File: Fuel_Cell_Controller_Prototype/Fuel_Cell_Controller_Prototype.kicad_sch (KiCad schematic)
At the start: 43 parts, among them J3 6POS MOLEX, Q1 NMOS, Q2 NMOS, U3 MAX14572, U4 MAX14572, U6 SHT31-DIS, U7 BUF602xD, U8 BUF602xD

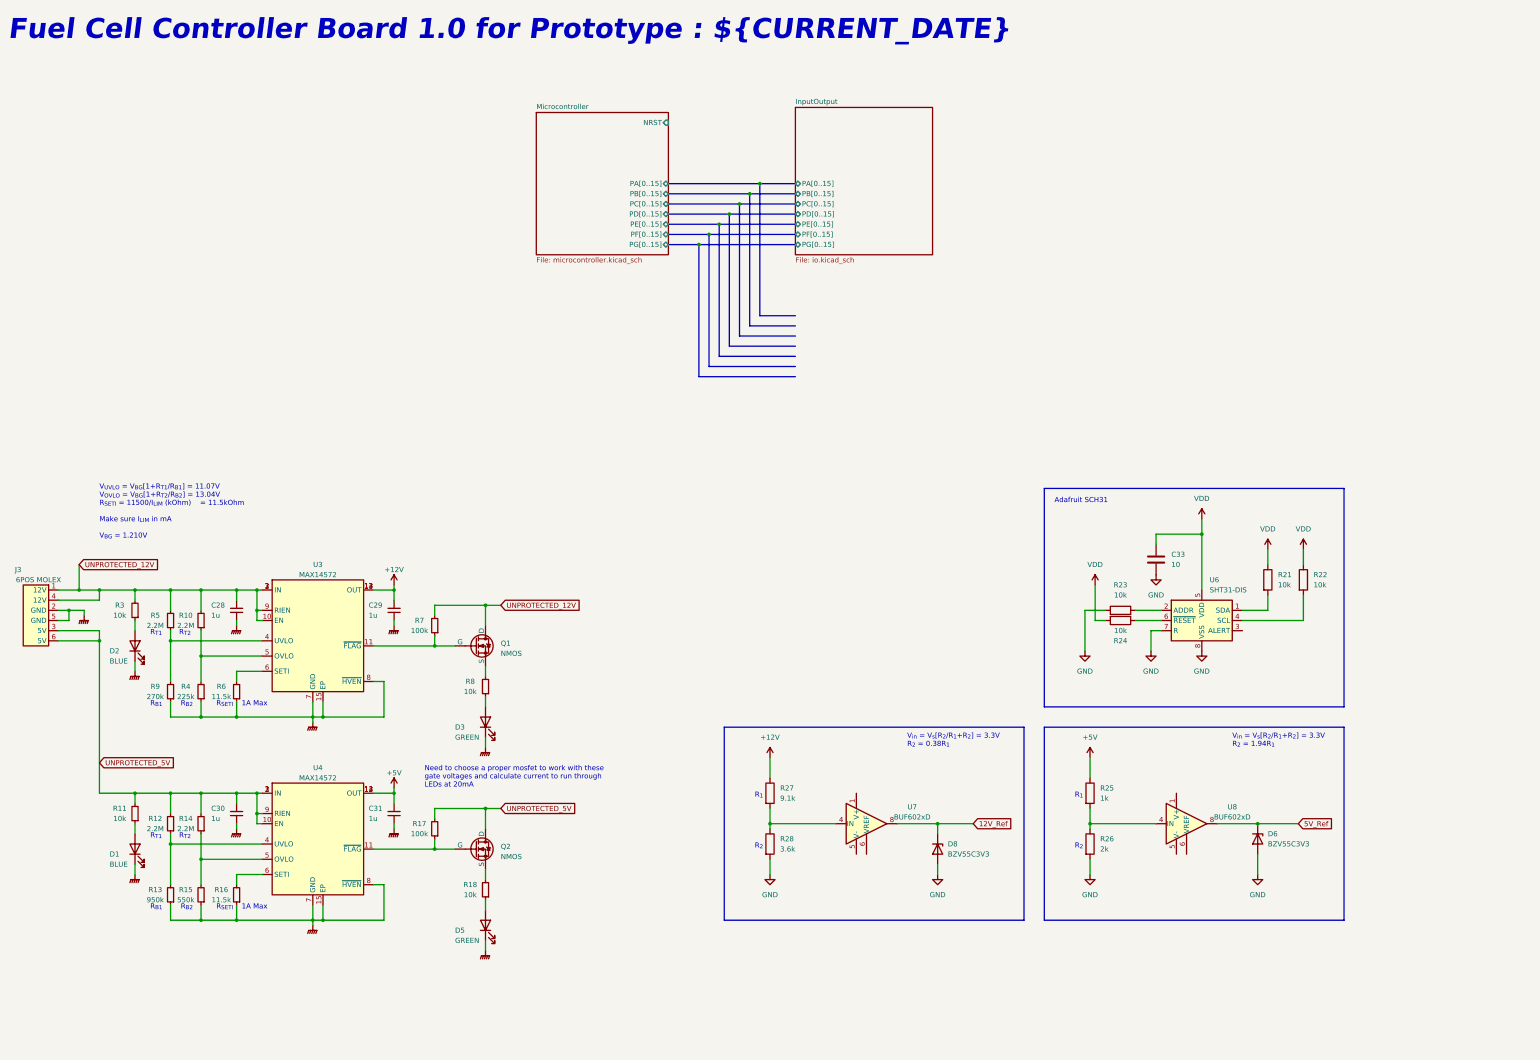
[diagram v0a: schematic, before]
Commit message: Update - Mikael
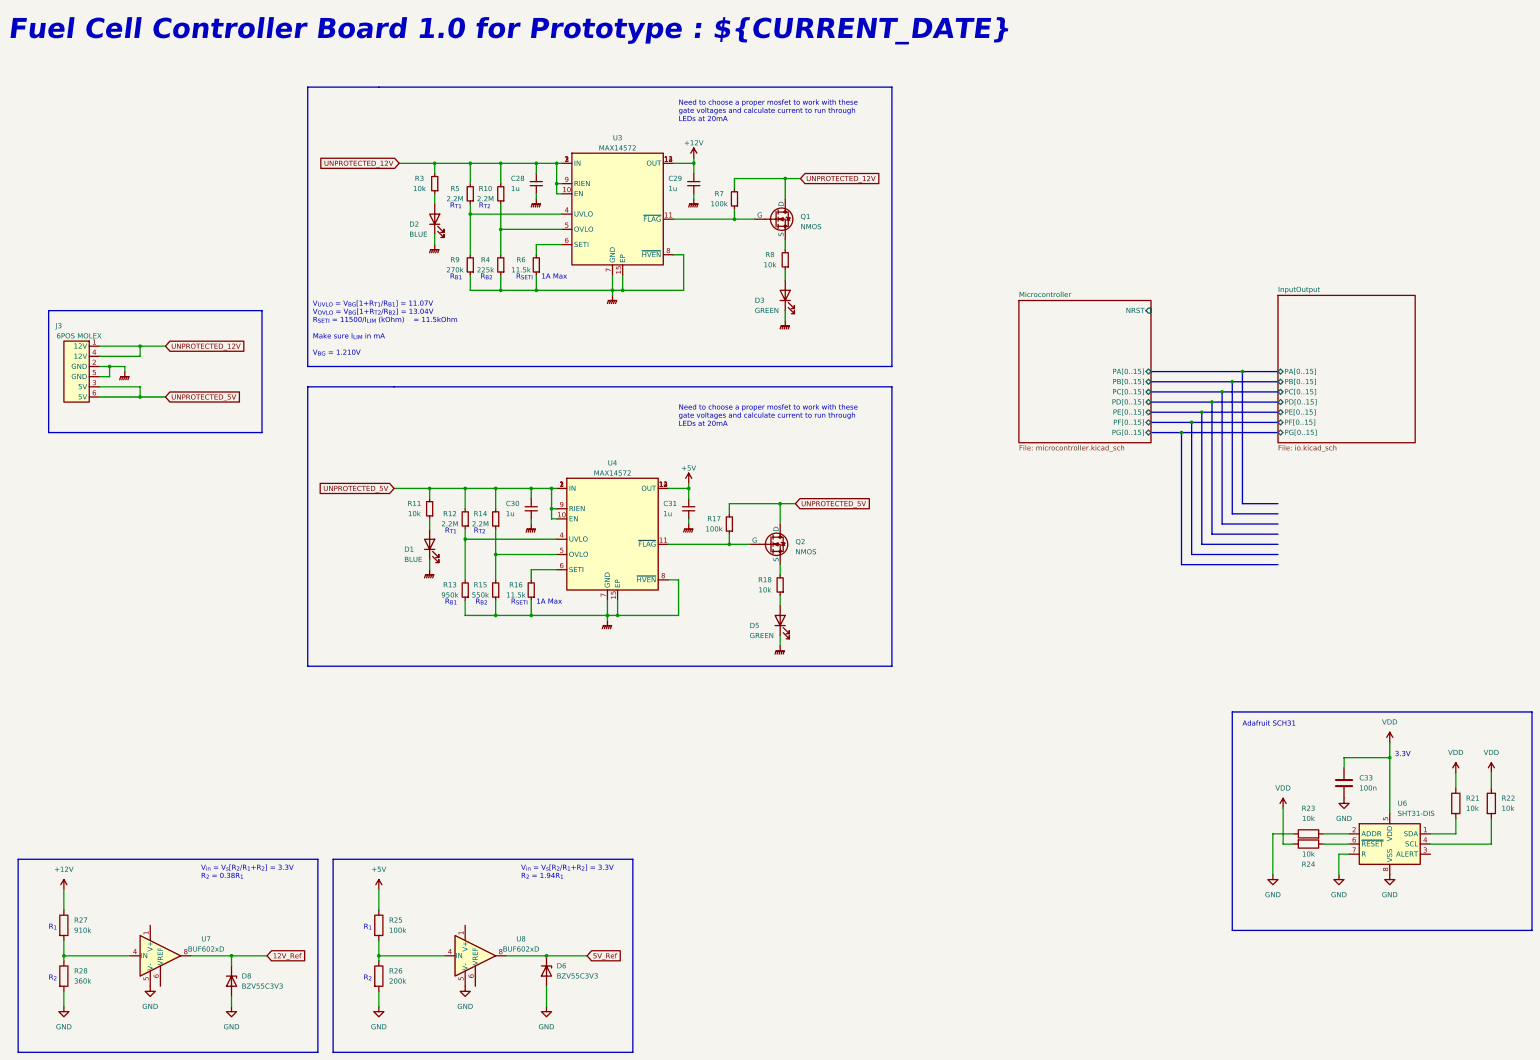
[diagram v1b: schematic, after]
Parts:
- C33: value 10 -> 100n
- R25: value 1k -> 100k
- R26: value 2k -> 200k
- R27: value 9.1k -> 910k
- R28: value 3.6k -> 360k
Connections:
- net GND: now also U7.5 (V-), U8.5 (V-)
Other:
- note added: "3.3V"
- moved on the sheet: C28, C29, C30, C31, C33, D1, D2, D3, D5, D6, D8, J3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
